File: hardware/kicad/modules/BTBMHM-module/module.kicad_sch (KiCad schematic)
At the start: 41 parts, among them J1 MOD_CONN, J10 MOD_CONN, J11 MOD_CONN, J12 MOD_CONN, J13 MOD_CONN, J14 MOD_CONN, J15 MOD_CONN, J16 MOD_CONN, J17 MOD_CONN, J18 MOD_CONN, J19 MOD_CONN, J2 MOD_CONN, J20 MOD_CONN, J21 MOD_CONN, J22 MOD_CONN, J3 MOD_CONN, J4 MOD_CONN, J5 MOD_CONN, J6 MOD_CONN, J7 MOD_CONN, J8 MOD_CONN, J9 MOD_CONN, SW2 EVP-AKE31A

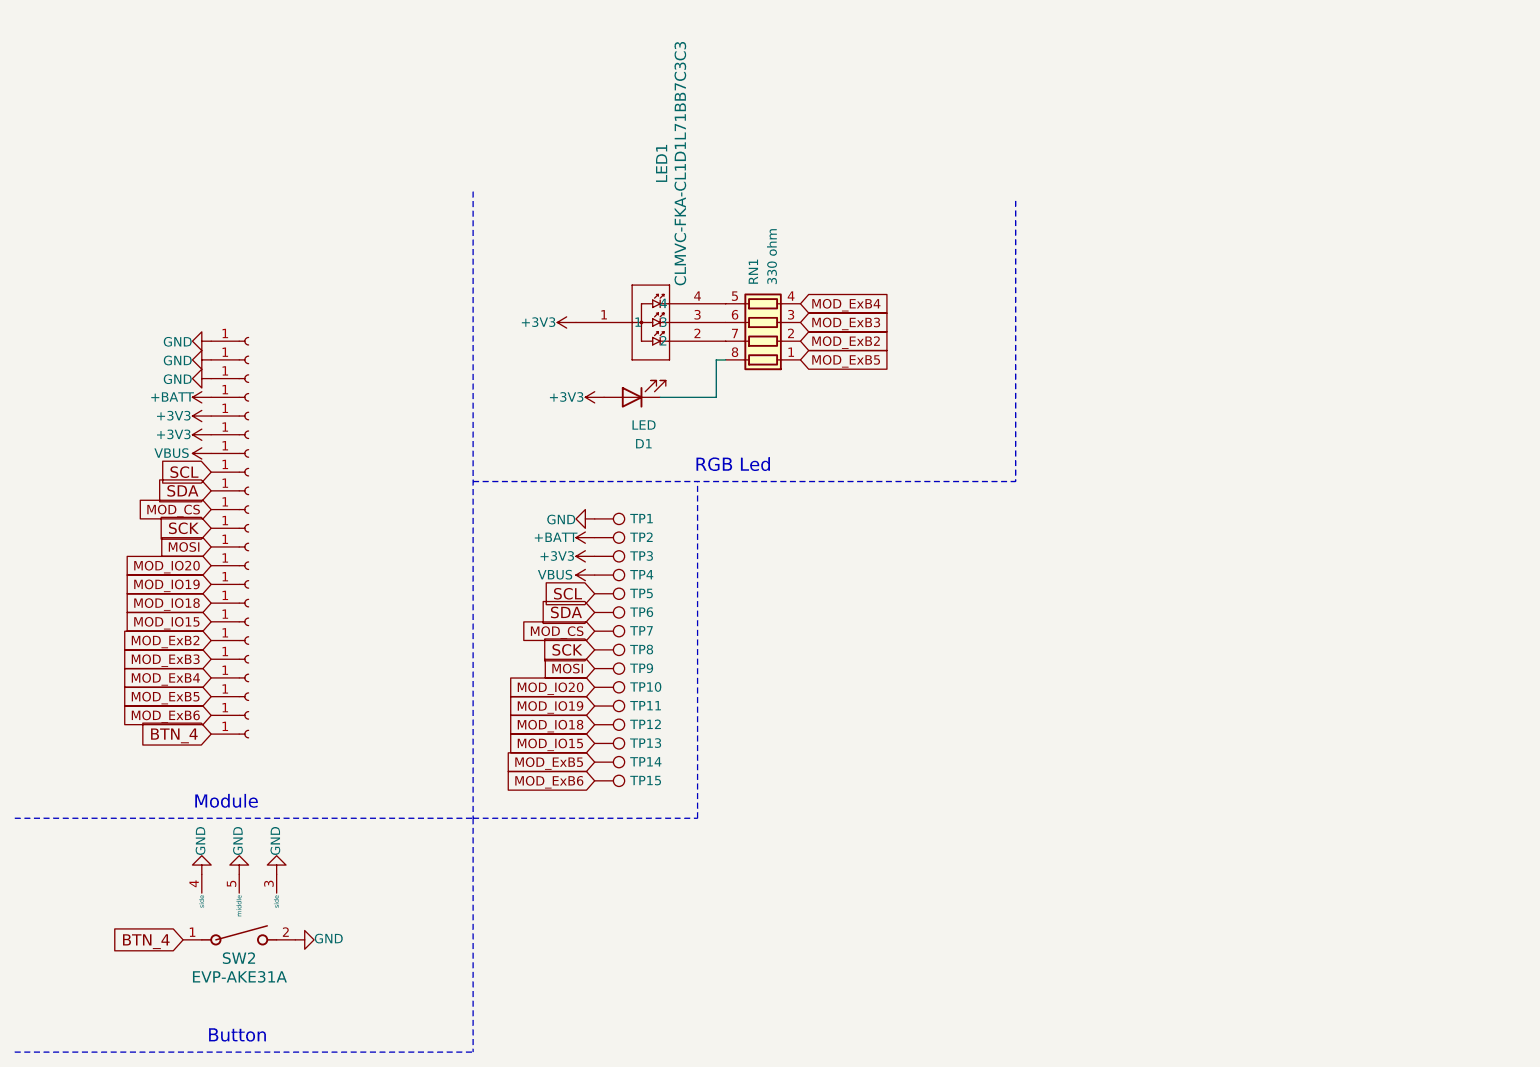
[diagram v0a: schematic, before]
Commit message: add new module
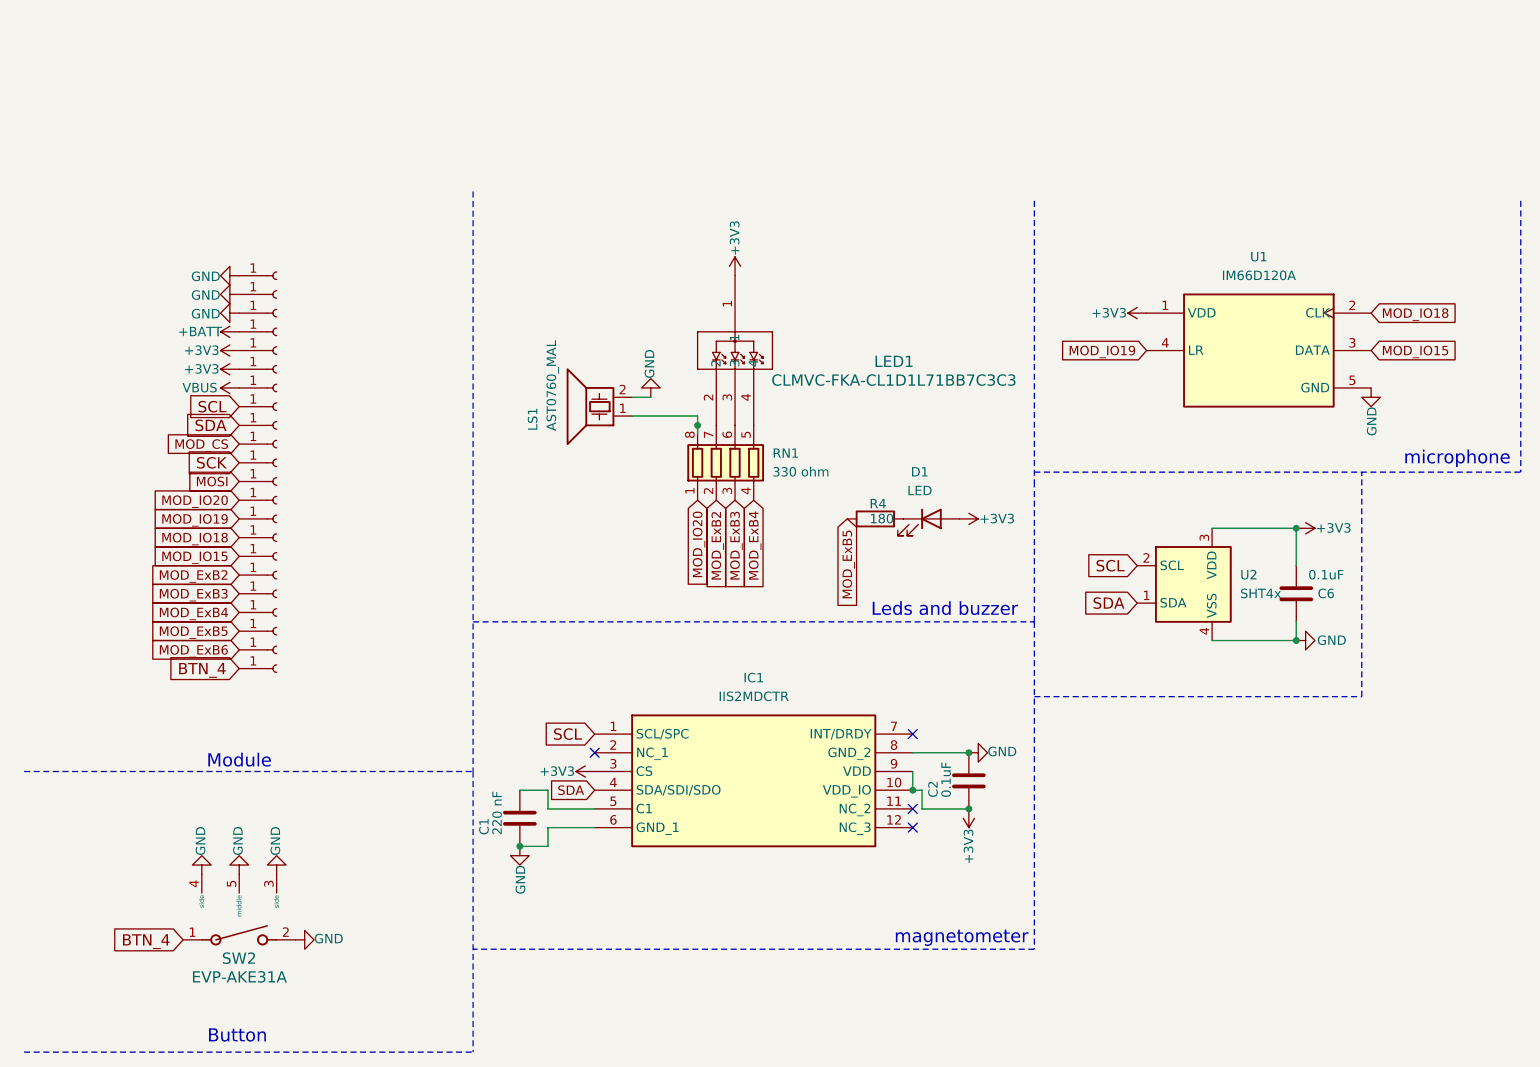
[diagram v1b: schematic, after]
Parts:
- removed TP1, TP10, TP11, TP12, TP13, TP14, TP15, TP2, TP3, TP4, TP5, TP6, TP7, TP8, TP9: TestPoint, Yatchy:TestPoint_THTPad_D1.0mm_Drill0.5mm, symbol Yatchy:TestPoint
- added C1: 220 nF, Capacitor_SMD:C_0603_1608Metric, symbol Watchy:C
- added C2: 0.1uF, Capacitor_SMD:C_0603_1608Metric, symbol Watchy:C
- added C6: 0.1uF, Capacitor_SMD:C_0603_1608Metric, symbol clock:C
- added IC1: IIS2MDCTR, Yatchy:BOSCH_LGA-12, symbol IIS2MDCTR:IIS2MDCTR
- added LS1: AST0760_MAL, Yatchy:AST0760_MAL, symbol Device:Speaker_Crystal
- added R4: 180, Resistor_SMD:R_0402_1005Metric, symbol Watchy:R
- added U1: IM66D120A, Yatchy:IFX-PG-TLGA-5-6-V, symbol IM66D120A:IM66D120A
- added U2: SHT4x, Yatchy:Sensirion_DFN-4_1.5x1.5mm_P0.8mm_SHT4x_NoCentralPad, symbol Sensor_Humidity:SHT4x
- RN1: footprint Yatchy:R_Array_Concave_4x0402 -> Resistor_SMD:R_Array_Concave_4x0402
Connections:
- net +3V3: now also C2.2, C6.2, IC1.10 (VDD_IO), IC1.3 (CS), IC1.9 (VDD), U1.1 (VDD), U2.3 (VDD)
- net GND: now also C1.2, C2.1, C6.1, IC1.6 (GND_1), IC1.8 (GND_2), LS1.2, U1.5 (GND), U2.4 (VSS)
- net MOD_ExB5: now also R4.1; no longer RN1.1 (R1.1)
- net MOD_IO15: now also U1.3 (DATA)
- net MOD_IO18: now also U1.2 (CLK)
- net MOD_IO19: now also U1.4 (LR)
- net MOD_IO20: now also RN1.1 (R1.1)
- net SCL: now also IC1.1 (SCL/SPC), U2.2 (SCL)
- net SDA: now also IC1.4 (SDA/SDI/SDO), U2.1 (SDA)
- net at D1.1 (K): now also R4.2; no longer RN1.8 (R1.2)
- new net: C1.1, IC1.5 (C1)
- new net: LS1.1, RN1.8 (R1.2)
- no-connect marks 0 -> 4
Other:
- note added: "Leds and buzzer"
- note added: "magnetometer"
- note added: "microphone"
- note removed: "RGB Led"
- moved on the sheet: D1, LED1, RN1
